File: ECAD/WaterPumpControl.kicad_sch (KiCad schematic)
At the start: 2 parts, among them U2 NCE3018AS, U9 NCE3018AS

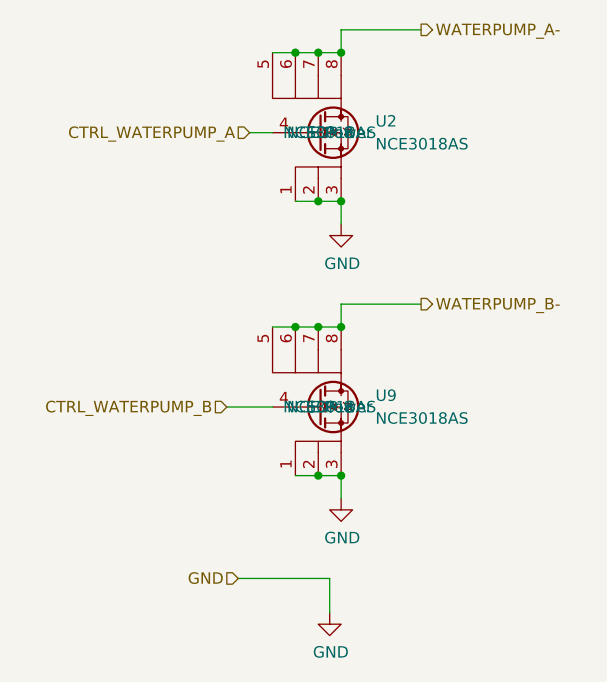
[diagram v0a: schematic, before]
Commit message: adding production and step files
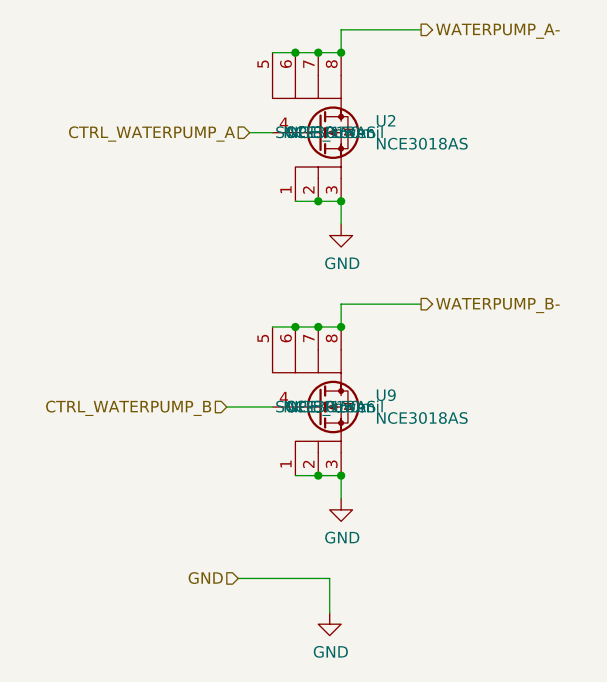
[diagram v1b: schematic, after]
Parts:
- U2, U9: Package SOP-8 -> SOP-8_150mil
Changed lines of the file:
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@@
     )
     (property "Manufacturer Number" "NCE3018AS" (id 4) (at 152.4 81.28 0))
-    (property "Package" "SOP-8" (id 5) (at 152.4 81.28 0))
+    (property "Package" "SOP-8_150mil" (id 5) (at 152.4 81.28 0))
     (property "Manufacturer" "NCE Power" (id 6) (at 152.4 81.28 0))
     (pin "5")
@@
     )
     (property "Manufacturer Number" "NCE3018AS" (id 4) (at 152.4 111.76 0))
-    (property "Package" "SOP-8" (id 5) (at 152.4 111.76 0))
+    (property "Package" "SOP-8_150mil" (id 5) (at 152.4 111.76 0))
     (property "Manufacturer" "NCE Power" (id 6) (at 152.4 111.76 0))
     (pin "5")
